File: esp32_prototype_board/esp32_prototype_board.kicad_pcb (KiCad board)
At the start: 4 copper layers, 90 x 65 mm, 74 parts, among them J1 USB-C USB2 sink, J2 EXT 5V IN, J4 microSD SPI, J6 SPI EXP, J7 I2C EXP, J8 GPIO EXP, Q1 SS8050/MMBT3904, Q2 SS8050/MMBT3904, Q3 MMBT3904, SW1 EN/RST, SW2 BOOT, U1 CH340C, U2 AP2112K-3.3, U3 ESP32-WROOM-32E, U4 MAX98357A blue module

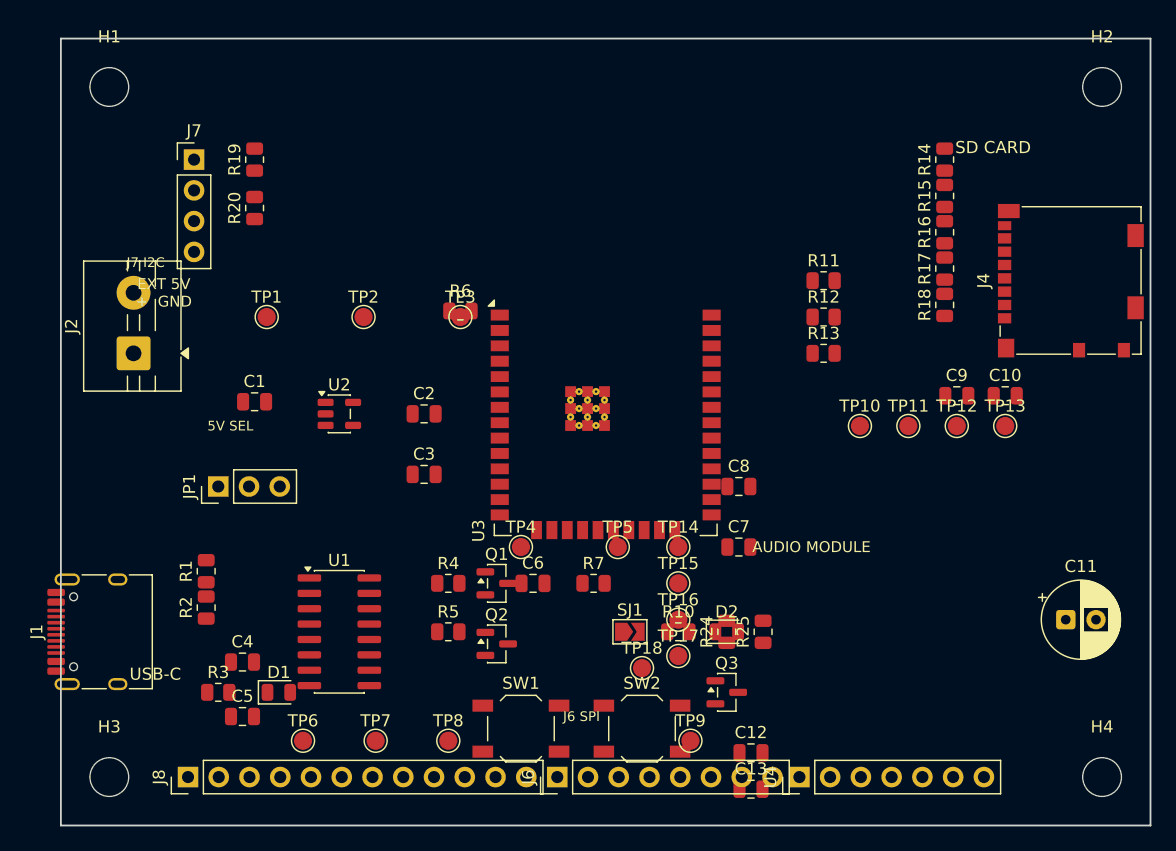
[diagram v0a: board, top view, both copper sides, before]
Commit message: adding final PCB files
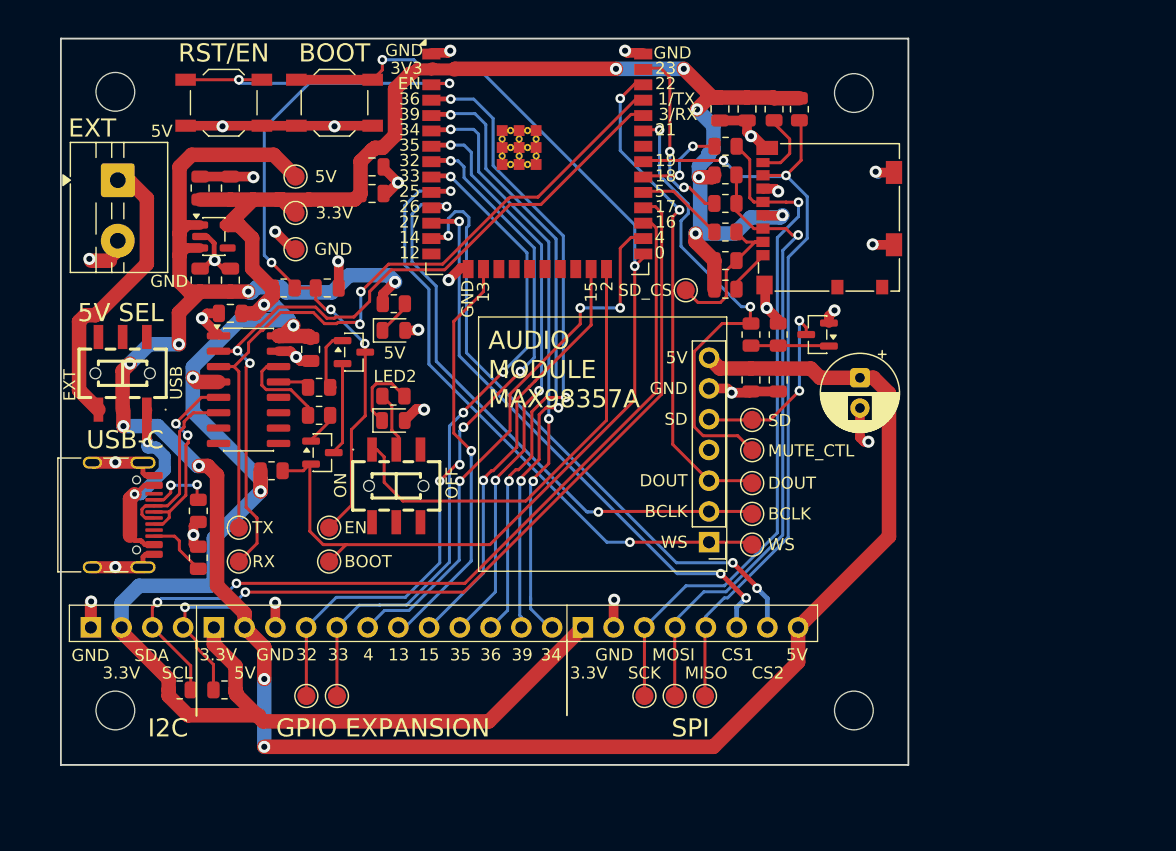
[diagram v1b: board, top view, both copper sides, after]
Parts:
- removed SJ1: GPIO2 LED EN, Jumper:SolderJumper-2_P1.3mm_Open_TrianglePad1.0x1.5mm
- added C14: 100nF, Capacitor_SMD:C_0805_2012Metric, F.Cu at (61.5, 72.0)
- added JP2: GPIO2 LED SW, SweetYaar:SW-SMD_MS-22D28-G020, F.Cu at (77.7, 89.0)
- H1, H2, H3, H4: value M3 -> M3 mounting hole
- JP1: value 5V source select -> 5V source switch; footprint Connector_PinHeader_2.54mm:PinHeader_1x03_P2.54mm_Vertical -> SweetYaar:SW-SMD_MS-22D28-G020
- moved SW2 57.6 mm to (72.6, 57.3)
- moved SW1 57.2 mm to (63.5, 57.3)
- moved R19 44.2 mm to (59.8, 105.8), turned to 0 degrees
- moved C7 42.1 mm to (75.7, 64.8)
- moved C8 40.2 mm to (75.7, 62.6)
- moved R20 39.9 mm to (63.5, 105.8), turned to 180 degrees
- moved J7 39.6 mm to (52.5, 100.6), turned to 90 degrees
- moved R3 35.2 mm to (77.5, 73.9)
- moved C13 33.9 mm to (109.2, 80.2), turned to -90 degrees
- moved D2 32.6 mm to (77.5, 83.5)
- moved C10 31.9 mm to (106.7, 57.8), turned to -90 degrees
- moved D1 31.4 mm to (77.5, 76.1)
- moved C5 30.8 mm to (70.6, 77.7), turned to -90 degrees
- moved C12 30.8 mm to (107.0, 80.2), turned to -90 degrees
- moved C9 30.7 mm to (104.4, 57.8), turned to -90 degrees
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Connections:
- J1 pad A8: (no net) -> unconnected-(J1-SBU1-PadA8)
- J1 pad B8: (no net) -> unconnected-(J1-SBU2-PadB8)
- U1 pad 10: (no net) -> unconnected-(U1-DSR-Pad10)
- U1 pad 11: (no net) -> unconnected-(U1-RI-Pad11)
- U1 pad 12: (no net) -> unconnected-(U1-DCD-Pad12)
- U1 pad 7: (no net) -> unconnected-(U1-NC-Pad7)
- U1 pad 8: (no net) -> unconnected-(U1-NC-Pad8)
- U1 pad 9: (no net) -> unconnected-(U1-CTS-Pad9)
- U2 pad 4: (no net) -> unconnected-(U2-NC-Pad4)
- U3 pad 14: (no net) -> unconnected-(U3-GPIO12-Pad14)
- U3 pad 17: (no net) -> unconnected-(U3-NC/SD2-Pad17)
- U3 pad 18: (no net) -> unconnected-(U3-NC/SD3-Pad18)
- U3 pad 19: (no net) -> unconnected-(U3-NC/CMD-Pad19)
- U3 pad 20: (no net) -> unconnected-(U3-NC/CLK-Pad20)
- U3 pad 21: (no net) -> unconnected-(U3-NC/SD0-Pad21)
- U3 pad 22: (no net) -> unconnected-(U3-NC/SD1-Pad22)
- U3 pad 32: (no net) -> unconnected-(U3-NC-Pad32)
- U4 pad 4: (no net) -> unconnected-(U4-GAIN-Pad4)
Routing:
- net /3V3: track 0.00 -> 212.8 mm, vias 0 -> 10
- net /5V_SYS: track 0.00 -> 182.9 mm, vias 0 -> 8
- net /GND: track 0.00 -> 98.0 mm, vias 0 -> 29
- net /BOOT: track 0.00 -> 93.0 mm, vias 0 -> 2
- net /I2C_SDA: track 0.00 -> 71.9 mm, vias 0 -> 2
- net /I2C_SCL: track 0.00 -> 71.3 mm, vias 0 -> 2
- net /EN: track 0.00 -> 69.7 mm, vias 0 -> 5
- net /SD_MISO: track 0.00 -> 67.2 mm, vias 0 -> 2
- net /UART0_RX: track 0.00 -> 63.8 mm, vias 0 -> 2
- net /UART0_TX: track 0.00 -> 61.0 mm, vias 0 -> 2
- net /GPIO32: track 0.00 -> 60.4 mm, vias 0 -> 5
- net /SD_SCK: track 0.00 -> 56.9 mm, vias 0 -> 1
- net /GPIO33: track 0.00 -> 56.0 mm, vias 0 -> 3
- net /GPIO36: track 0.00 -> 54.0 mm, vias 0 -> 3
- net /I2S_WS: track 0.00 -> 52.7 mm, vias 0 -> 2
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- added copper zone on In1.Cu, net /GND
- added copper zone on In2.Cu, net /GND
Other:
- board size 90 x 65 mm -> 70 x 60 mm
- board text added: "0"
- board text added: "1/TX"
- board text added: "12"
- board text added: "13"
- board text added: "14"
- board text added: "15"
- board text added: "16"
- board text added: "17"
- board text added: "18"
- board text added: "19"
- board text added: "2"
- board text added: "21"
- board text added: "22"
- board text added: "23"
- board text added: "25"
- board text added: "26"
- board text added: "27"
- board text added: "3.3V"
- board text added: "3/RX"
- board text added: "32"
- board text added: "33"
- board text added: "34"
- board text added: "35"
- board text added: "36"
- board text added: "39"
- board text added: "3V3"
- board text added: "4"
- board text added: "5"
- board text added: "5V"
- board text added: "AUDIO MODULE MAX98357A"
- board text added: "BCLK"
- board text added: "BOOT"
- board text added: "CS1"
- board text added: "CS2"
- board text added: "DOUT"
- board text added: "EN"
- board text added: "ESP32 Dev Board (by Zach Moshe)"
- board text added: "EXT"
- board text added: "GND"
- board text added: "GPIO EXPANSION"
- board text added: "I2C"
- board text added: "LED2"
- board text added: "MISO"
- board text added: "MOSI"
- board text added: "MUTE_CTL"
- board text added: "OFF"
- board text added: "ON"
- board text added: "RST/EN"
- board text added: "RX"
- board text added: "Rev A first placement: 70mm x 60mm"
- board text added: "SCK"
- board text added: "SCL"
- board text added: "SD"
- board text added: "SDA"
- board text added: "SD_CS"
- board text added: "SPI"
- board text added: "TX"
- board text added: "USB"
- board text added: "WS"
- board text removed: "AUDIO MODULE"
- board text removed: "ESP32 antenna keepout: no copper, traces, parts, screws, or wires"
- board text removed: "EXT 5V + GND"
- board text removed: "J6 SPI"
- board text removed: "J7 I2C"
- board text removed: "Rev A first placement: 90mm x 65mm"
- board text removed: "SD CARD"
